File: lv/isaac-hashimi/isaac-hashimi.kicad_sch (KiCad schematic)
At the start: 5 parts, among them U1 LMV393

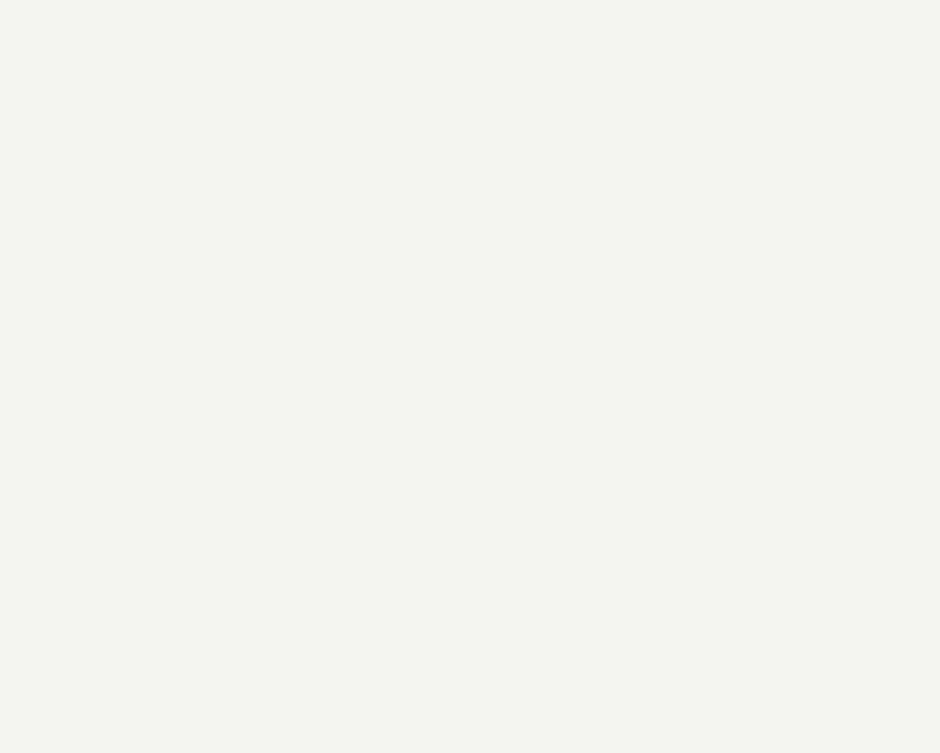
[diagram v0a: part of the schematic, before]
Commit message: Add current comparator
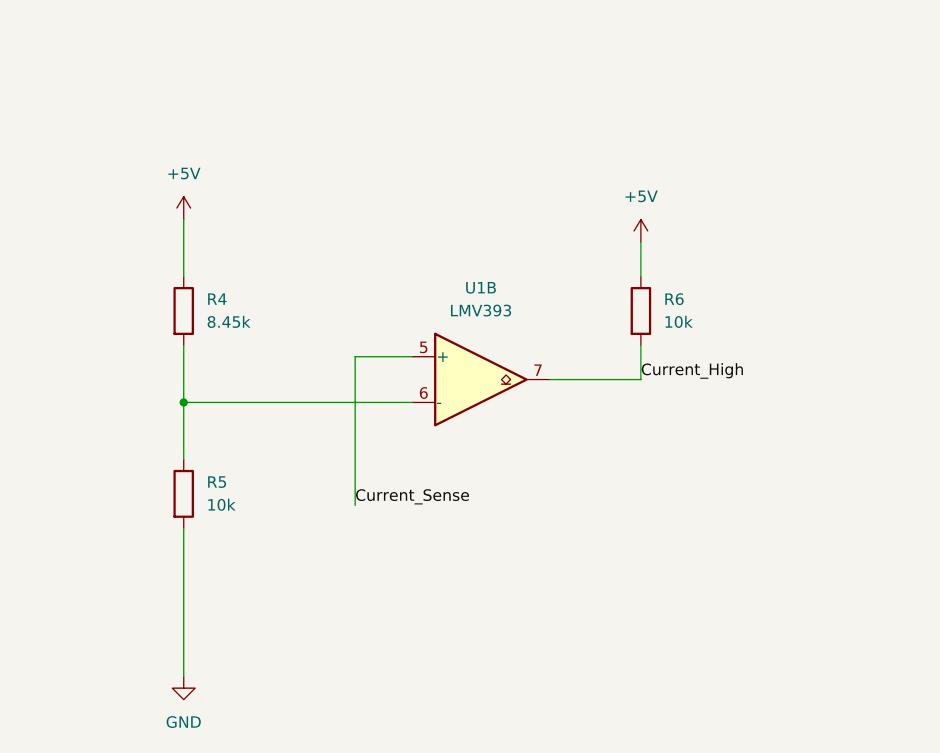
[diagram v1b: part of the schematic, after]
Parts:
- added R4: 8.45k, Resistor_THT:R_Array_SIP4, symbol Device:R
- added R5, R6: 10k, Resistor_THT:R_Array_SIP4, symbol Device:R
- added unit 2 of U1
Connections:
- net +5V: now also R4.1, R6.1
- net GND: now also R5.2
- new net: R4.2, R5.1, U1.6 (-)
- new net Current_High: R6.2, U1.7
- new net Current_Sense: U1.5 (+)
